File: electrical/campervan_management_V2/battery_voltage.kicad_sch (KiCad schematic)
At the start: 47 parts, among them U10 LM358DR2G, U11 LM358DR2G, U14 HCNR200-500E, U15 LM358DR2G, U4 HCNR200-500E, U6 LM358DR2G, U7 LM358DR2G, U9 HCNR200-500E

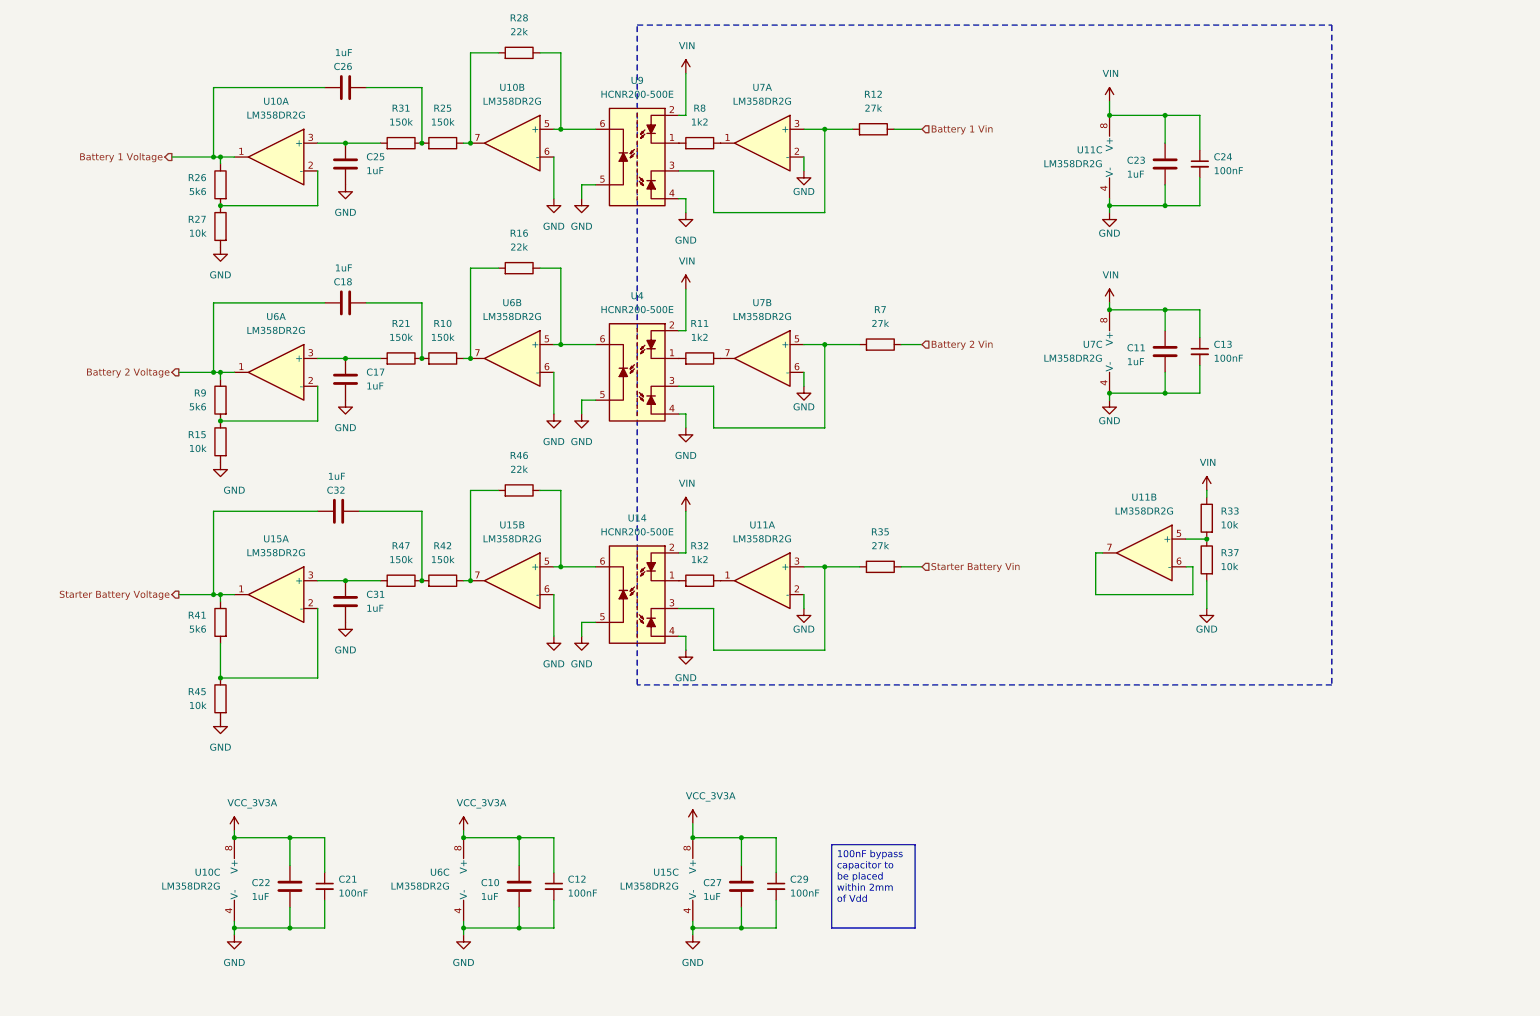
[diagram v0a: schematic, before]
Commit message: updated
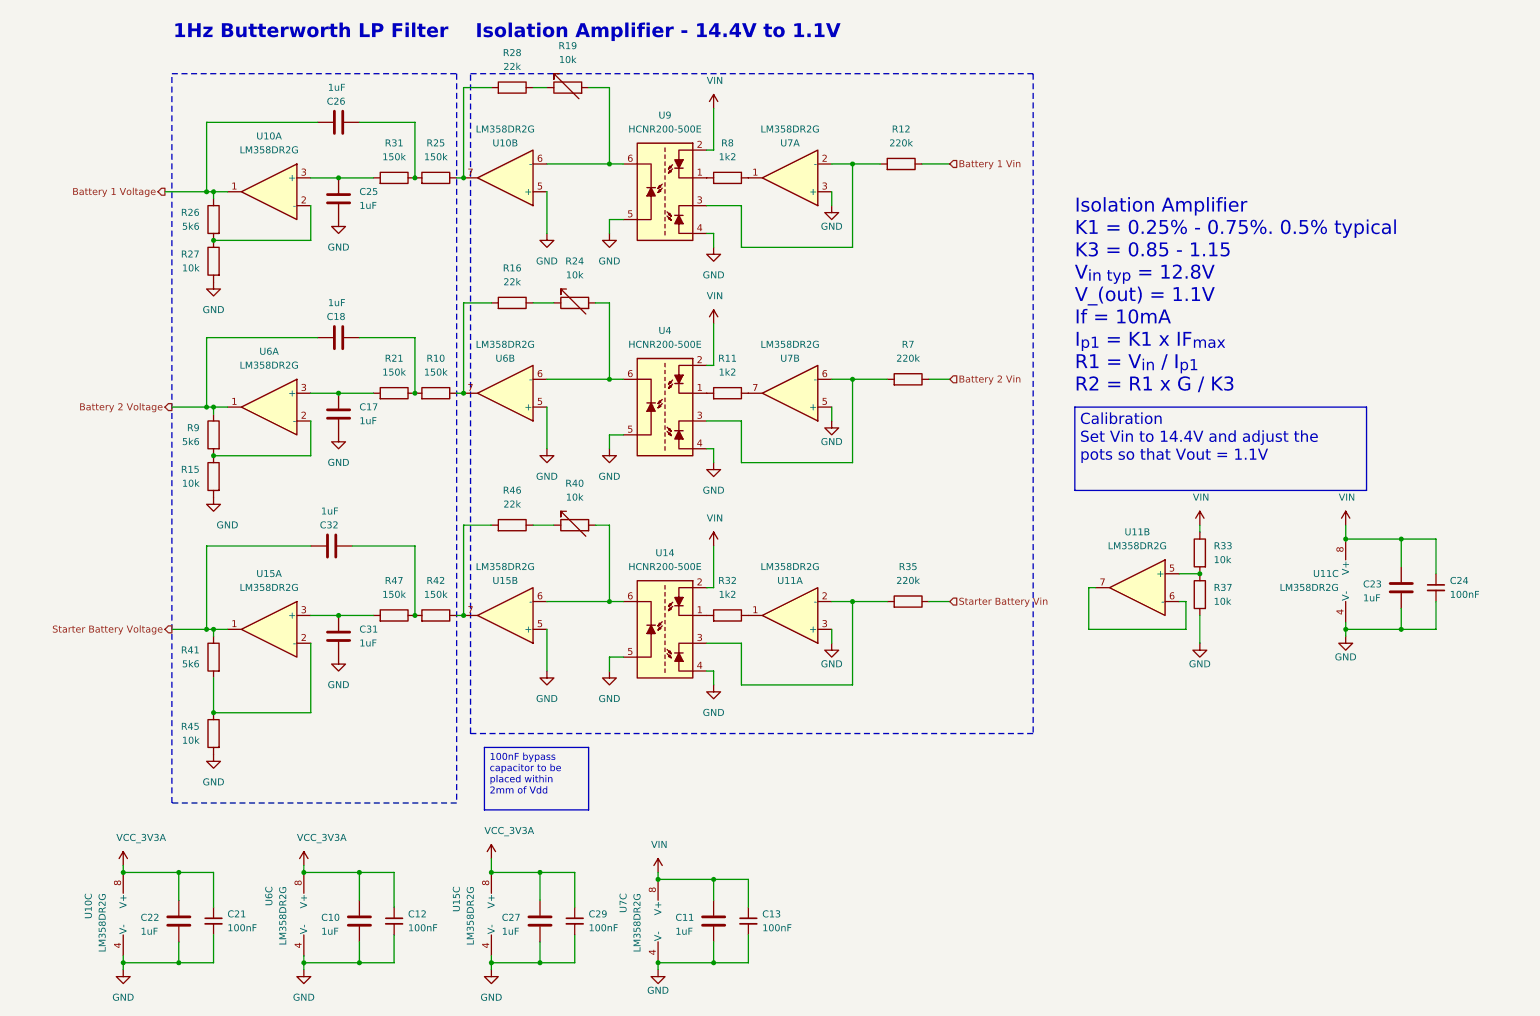
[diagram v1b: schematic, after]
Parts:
- added R19, R24, R40: 10k, Potentiometer_THT:Potentiometer_Bourns_3296W_Vertical, symbol Device:R_Variable
- R12, R35, R7: value 27k -> 220k
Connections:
- net GND: now also U10.5 (+), U11.3 (+), U15.5 (+), U6.5 (+), U7.3 (+), U7.5 (+); no longer U10.6 (-), U11.2 (-), U15.6 (-), U6.6 (-), U7.2 (-), U7.6 (-)
- net at R35.2, U14.3: now also U11.2 (-); no longer U11.3 (+)
- net at R7.2, U4.3: now also U7.6 (-); no longer U7.5 (+)
- net at R12.2, U9.3: now also U7.2 (-); no longer U7.3 (+)
- new net: R40.1, R46.1
- new net: R40.2, U14.6, U15.6 (-)
- new net: R24.2, U4.6, U6.6 (-)
- new net: R16.1, R24.1
- new net: R19.2, U10.6 (-), U9.6
- new net: R19.1, R28.1
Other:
- note added: "1Hz Butterworth LP Filter"
- note added: "Isolation Amplifier - 14.4V to 1.1V"
- note added: "Isolation Amplifier K1 = 0.25% - 0.75%. 0.5% typical K3 = 0.85 - 1.15 V_{in typ} = 12.8V V_(out) = 1.1V If = 10mA I_{p1} = K1 x IF_{max} R1 = V_{in} / I_{p1} R2 = R1 x G / K3"
- moved on the sheet: C10, C11, C12, C13, C17, C18, C21, C22, C23, C24, C25, C26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
